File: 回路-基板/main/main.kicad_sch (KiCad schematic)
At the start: 49 parts, among them J1 Conn_01x07_Pin, Q1 PMOS, Q2 NMOS, Q3 PMOS, Q4 NMOS, SW1 SW_SPDT, SW2 SW_Push, SW3 SW_Push, SW4 SW_Push, SW5 SW_Push, SW6 SW_Push, U1 TWE-L-WX, U2 LM1117MP-3.3

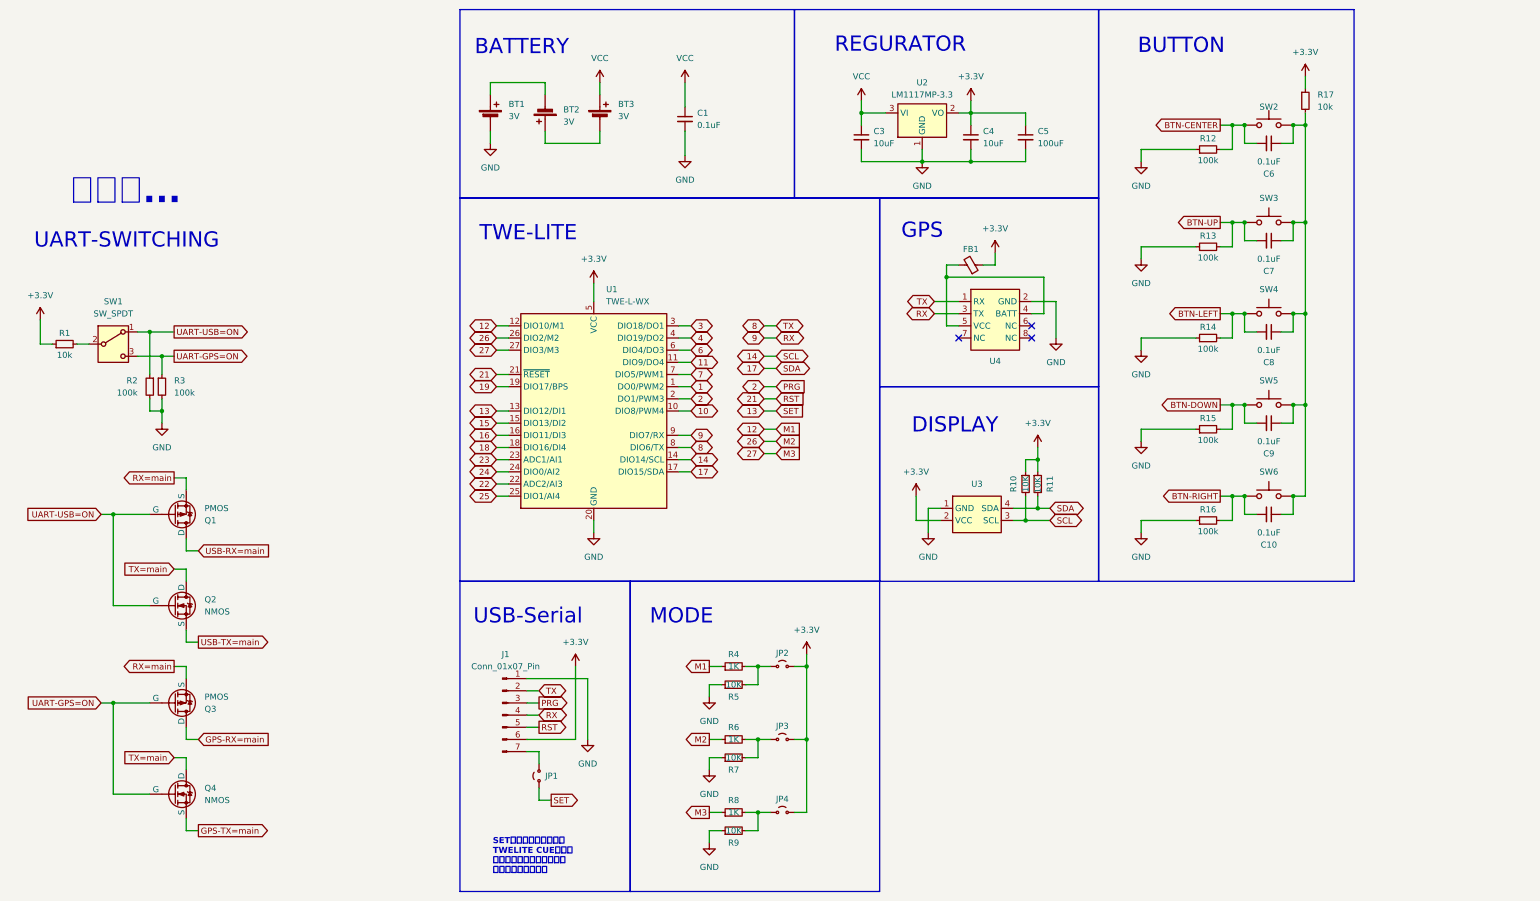
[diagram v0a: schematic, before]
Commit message: 回路図/PCB両方一応完成した
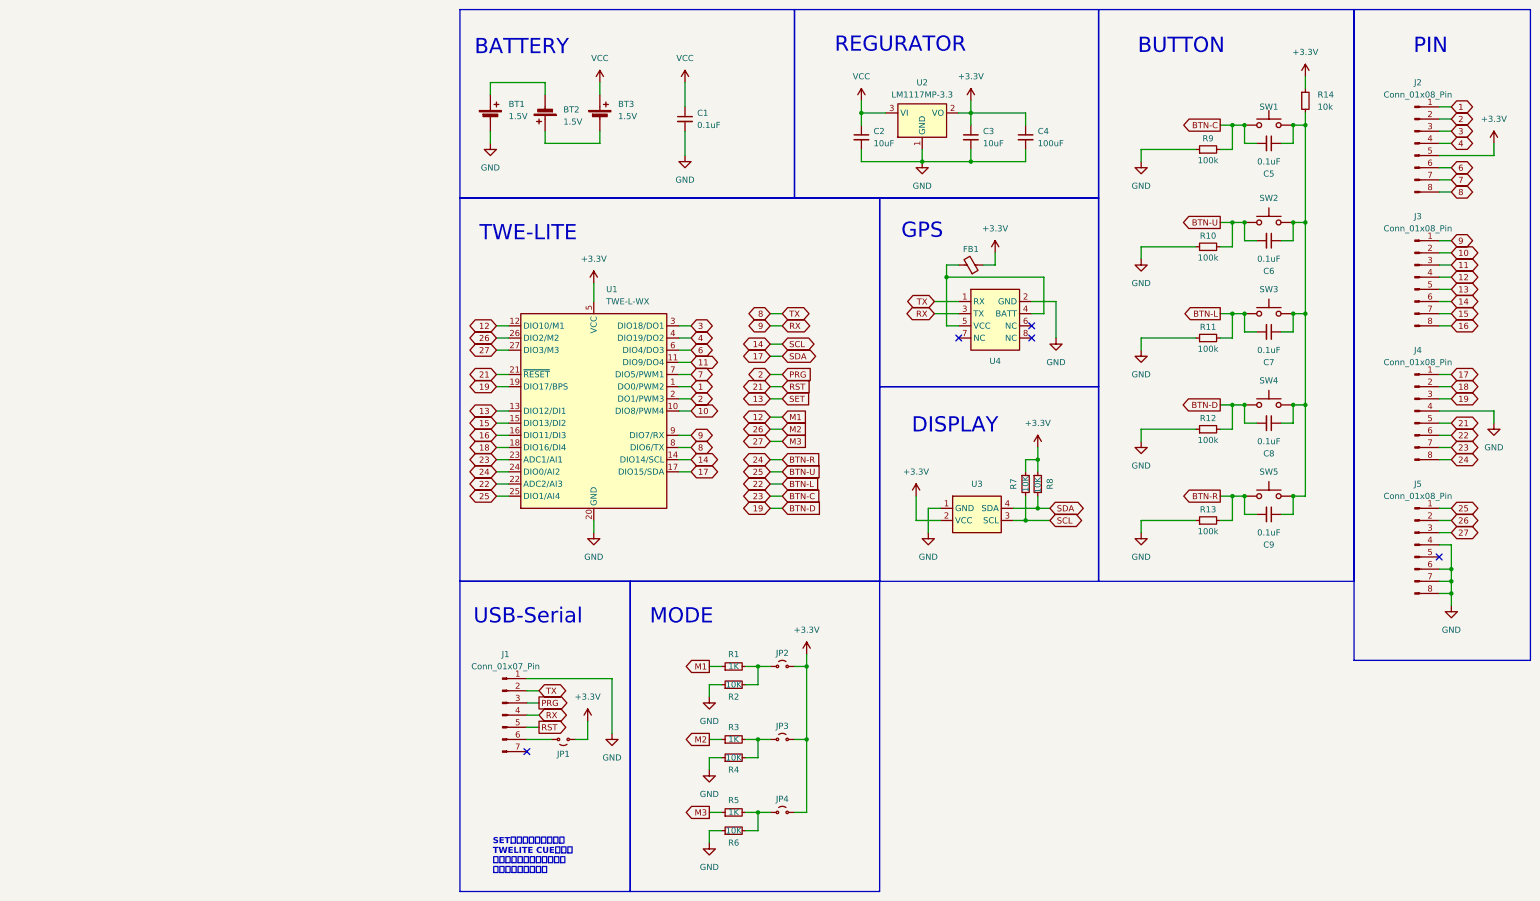
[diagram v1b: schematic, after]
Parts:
- removed Q1, Q3: PMOS, symbol Simulation_SPICE:PMOS
- removed Q2, Q4: NMOS, symbol Simulation_SPICE:NMOS
- removed R1: 10k, Resistor_SMD:R_0805_2012Metric, symbol Device:R_Small
- removed R2, R3: 100k, Resistor_SMD:R_0805_2012Metric, symbol Device:R_Small
- removed SW1: SW_SPDT, @2024-cansat:SS12D01G4, symbol Switch:SW_SPDT
- added J2, J3, J4, J5: Conn_01x08_Pin, @2024-cansat:Pin-Extender, symbol Connector:Conn_01x08_Pin
- BT1, BT2, BT3: value 3V -> 1.5V; footprint @2024-cansat:BHSD-2032-SM -> @2024-cansat:AAA-holder
- J1: footprint Connector_PinHeader_2.54mm:PinHeader_1x07_P2.54mm_Horizontal -> Connector_PinSocket_2.54mm:PinSocket_1x07_P2.54mm_Vertical
- renumbered C3 to C2, C4 to C3, C5 to C4, C6 to C5, C7 to C6, C8 to C7, C9 to C8, C10 to C9, R4 to R1, R13 to R10, R14 to R11, R15 to R12, R16 to R13, R17 to R14, R5 to R2, R6 to R3, R7 to R4, R8 to R5, R9 to R6, R10 to R7, R11 to R8, R12 to R9, SW2 to SW1, SW3 to SW2, SW4 to SW3, SW5 to SW4, SW6 to SW5
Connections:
- net BTN-CENTER is gone; now on net 23: C5.2, R9.2, SW1.1
- net BTN-DOWN is gone; now on net 19: C8.2, R12.2, SW4.1
- net BTN-LEFT is gone; now on net 22: C7.2, R11.2, SW3.1
- net BTN-RIGHT is gone; now on net 24: C9.2, R13.2, SW5.1
- net BTN-UP is gone; now on net 25: C6.2, R10.2, SW2.1
- net +3.3V: now also JP1.1 (A), J2.5 (Pin_5); no longer J1.6 (Pin_6)
- net 1: now also J2.1 (Pin_1)
- net 10: now also J3.2 (Pin_2)
- net 11: now also J3.3 (Pin_3)
- net 12: now also J3.4 (Pin_4)
- net 13: now also J3.5 (Pin_5); no longer JP1.1 (A)
- net 14: now also J3.6 (Pin_6)
- net 15: now also J3.7 (Pin_7)
- net 16: now also J3.8 (Pin_8)
- net 17: now also J4.1 (Pin_1)
- net 18: now also J4.2 (Pin_2)
- net 19: now also J4.3 (Pin_3)
- net 2: now also J2.2 (Pin_2)
- net 21: now also J4.5 (Pin_5)
- net 22: now also J4.6 (Pin_6)
- net 23: now also J4.7 (Pin_7)
- net 24: now also J4.8 (Pin_8)
- net 25: now also J5.1 (Pin_1)
- net 26: now also J5.2 (Pin_2)
- net 27: now also J5.3 (Pin_3)
- net 3: now also J2.3 (Pin_3)
- net 4: now also J2.4 (Pin_4)
- net 6: now also J2.6 (Pin_6)
- net 7: now also J2.7 (Pin_7)
- net 8: now also J2.8 (Pin_8)
- net 9: now also J3.1 (Pin_1)
- net GND: now also J4.4 (Pin_4), J5.4 (Pin_4), J5.6 (Pin_6), J5.7 (Pin_7), J5.8 (Pin_8)
- net at JP1.2 (B): now also J1.6 (Pin_6); no longer J1.7 (Pin_7)
- no-connect marks 3 -> 5
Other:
- note added: "PIN"
- note removed: "UART-SWITCHING"
- note removed: "考え中..."
